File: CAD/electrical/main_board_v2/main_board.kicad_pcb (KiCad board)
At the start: 2 copper layers, 125.2 x 61.2 mm, 70 parts, among them J1 Battery in, J10 I2C Motor, J13 RS485, J14 RS485, J3 Trigger, J301 USB_B, J302 UART PGM, J4 Side select, J7 I2C Peripheral, J8 I2C Peripheral, J9 I2C Motor, Q301 Q_NPN_BEC, Q302 Q_NPN_BEC, SW3 Input encoder, SW301 BOOT, SW302 RESET, U11 SRV05-4, U201 LM2576S-5, U202 AMS1117-3.3, U3 ESP32-WROOM-32, U301 SRV05-4, U302 CP2102N-Axx-xQFN28, U4 PCA9306DC1, U5 PCA9306DC1, U7 LCD-016N002L, U8 MAX485E, U9 SRV05-4

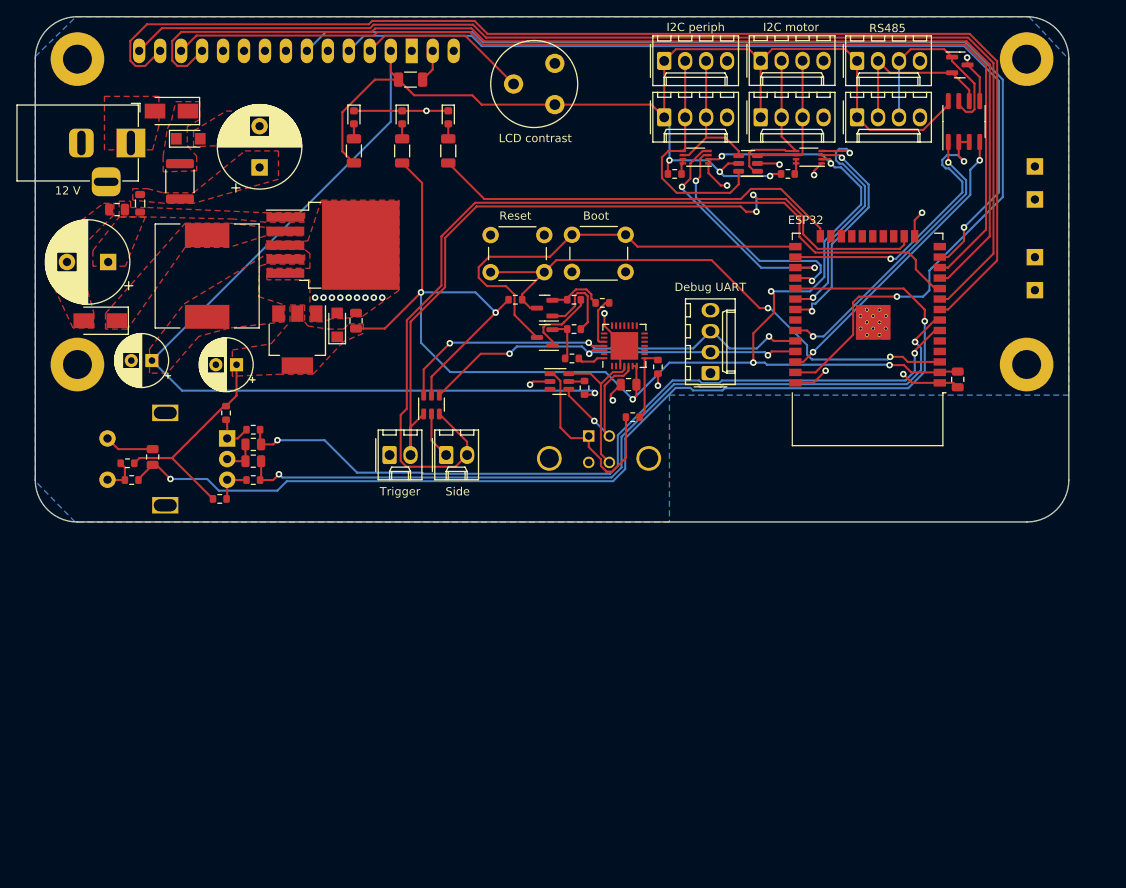
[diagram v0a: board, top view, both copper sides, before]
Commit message: Kicad CAD for mainboard and motorboard (final)
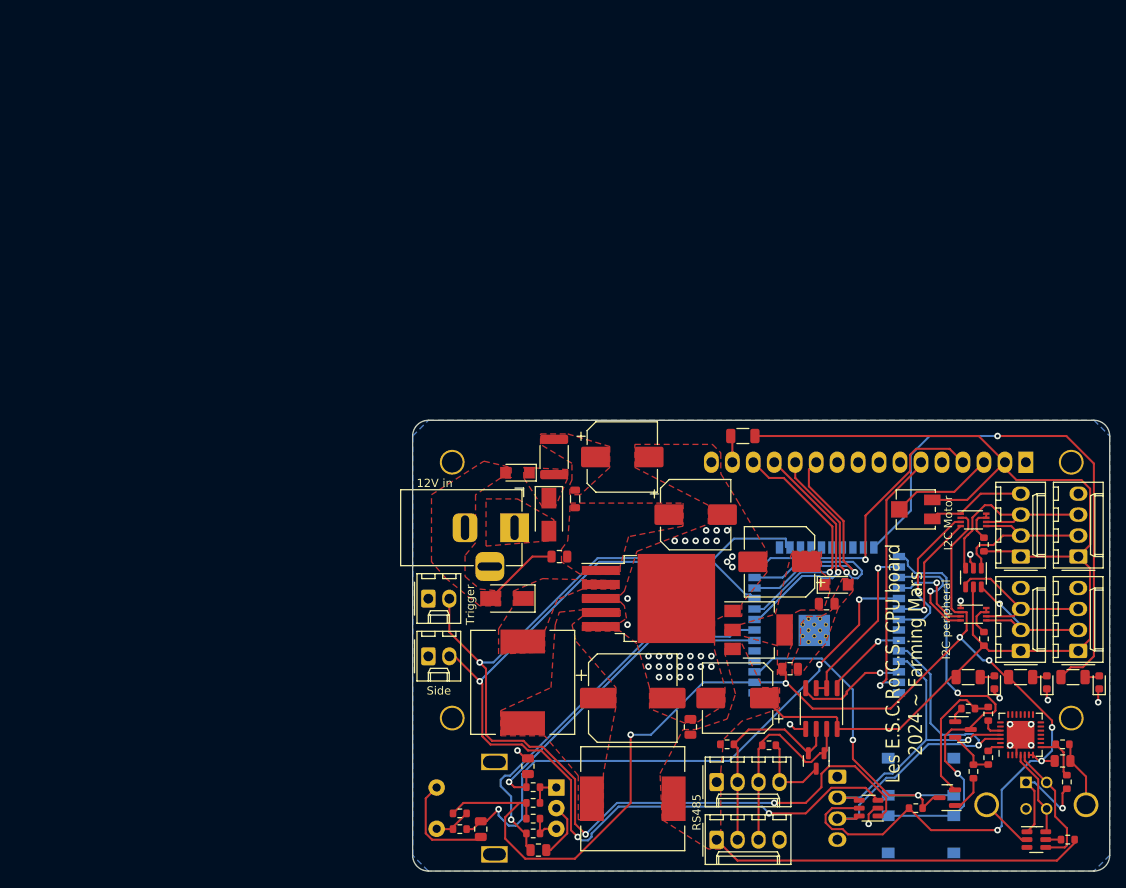
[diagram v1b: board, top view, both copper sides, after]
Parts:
- removed J302: UART PGM, Connector_Molex:Molex_KK-254_AE-6410-04A_1x04_P2.54mm_Vertical
- added C1: 100u, Capacitor_SMD:CP_Elec_8x10, F.Cu at (142.0, 100.1)
- added C2: 100n, Capacitor_SMD:C_0805_2012Metric, F.Cu at (136.3, 103.6)
- added J2: UART PGM, Connector_Molex:Molex_KK-254_AE-6410-04A_1x04_P2.54mm_Vertical, B.Cu at (154.1, 109.6)
- added L1: 10u, Inductor_SMD:L_12x12mm_H6mm, F.Cu at (129.3, 112.3)
- added R2: 1k, Resistor_SMD:R_0603_1608Metric, F.Cu at (140.7, 105.7)
- added R3: 1k, Resistor_SMD:R_0603_1608Metric, F.Cu at (145.8, 105.8)
- C201, C202: footprint Capacitor_THT:CP_Radial_D10.0mm_P5.00mm -> Capacitor_SMD:CP_Elec_8x10
- C204: value 10u -> 2000u; footprint Capacitor_THT:CP_Radial_D6.3mm_P2.50mm -> Capacitor_SMD:CP_Elec_10x10.5
- C205: value 10u -> 100u; footprint Capacitor_THT:CP_Radial_D6.3mm_P2.50mm -> Capacitor_SMD:CP_Elec_8x10
- R1: value 470 -> 300
- R10, R14, R9: value 470 -> 620
- R202, R4: value 100 -> 300
- R301: value 47k -> 82k
- R302: value 24k -> 36k
- R5, R6: value 100k -> 33k
- RV1: footprint Potentiometer_THT:Potentiometer_Piher_PT-10-V05_Vertical -> Potentiometer_SMD:Potentiometer_Bourns_3314J_Vertical
- SW301, SW302: footprint Button_Switch_THT:SW_PUSH_6mm -> Button_Switch_SMD:SW_Push_1P1T_NO_6x6mm_H9.5mm; moved to B.Cu
- U3: footprint RF_Module:ESP32-WROOM-32 -> RF_Module:ESP32-WROOM-32U; moved to B.Cu
- U7: footprint Display:LCD-016N002L -> Display:WC1602A
- moved D4 104.4 mm to (185.8, 98.2), turned to 90 degrees
- moved D205 103.9 mm to (179.5, 98.2), turned to 90 degrees
- moved D204 103.5 mm to (173.1, 98.2), turned to 90 degrees
- moved R4 99.0 mm to (182.6, 97.5), turned to 0 degrees
- moved R202 98.4 mm to (176.3, 97.5), turned to 0 degrees
- moved R201 98.0 mm to (169.9, 97.5), turned to 0 degrees
- moved J13 95.9 mm to (139.4, 117.2)
- moved U7 89.6 mm to (176.9, 71.5)
- moved D8 86.1 mm to (151.5, 107.7), turned to -90 degrees
- moved SW301 84.1 mm to (164.2, 116.6), turned to 180 degrees
- moved SW302 83.8 mm to (164.2, 109.6), turned to 180 degrees
- moved J8 83.5 mm to (176.3, 94.4), turned to 90 degrees
- moved J14 82.3 mm to (139.4, 110.3)
- moved J7 81.8 mm to (183.3, 94.4), turned to 90 degrees
- moved R306 80.1 mm to (182.0, 117.2), turned to 180 degrees
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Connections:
- C204 pad 1: +5V -> Net-(C204-Pad1)
- L201 pad 2: +5V -> Net-(C204-Pad1)
- U201 pad 4: +5V -> Net-(C204-Pad1)
- U3 pad 34: /UART_MOSI -> /UART_RX
- U3 pad 35: /UART_MISO -> /UART_TX
- U302 pad 25: /UART_MOSI -> /UART_TX
- U302 pad 26: /UART_MISO -> /UART_RX
- U9 pad 4: /UART_MISO -> /UART_TX
- U9 pad 6: /UART_MOSI -> /UART_RX
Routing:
- net /LCD_DB6: track 148.6 -> 29.3 mm, vias 0 -> 1
- net /LCD_DB7: track 138.6 -> 29.4 mm, vias 0 -> 1
- net /LCD_E: track 139.5 -> 31.5 mm
- net /LCD_DB4: track 137.5 -> 29.6 mm, vias 0 -> 1
- net /LCD_DB5: track 127.5 -> 32.9 mm, vias 0 -> 1
- net /LCD_RS: track 106.7 -> 36.3 mm
- net /INPUT_SW: track 129.5 -> 71.5 mm, vias 2 -> 3
- net +5V: track 241.9 -> 186.0 mm, vias 4 -> 0
- net /INPUT_A: track 96.3 -> 40.9 mm, vias 2 -> 1
- net /UART_MOSI: track 54.1 -> 0.00 mm, vias 3 -> 0
- net /INPUT_B: track 97.9 -> 48.4 mm, vias 2 -> 1
- net /UART_MISO: track 48.4 -> 0.00 mm, vias 3 -> 0
- net /UART_RX: track 0.00 -> 45.8 mm, vias 0 -> 1
- net /UART_TX: track 0.00 -> 37.2 mm, vias 0 -> 1
- net +3V3: track 210.7 -> 176.8 mm, vias 8 -> 7
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- added copper zone on F.Cu, net Net-(C204-Pad1)
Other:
- board size 125.2 x 61.2 mm -> 84.5 x 54.6 mm
- board text added: "12V in"
- board text added: "BOOT"
- board text added: "I2C Motor"
- board text added: "I2C peripheral"
- board text added: "Les E.S.C.Ro.C.S. CPU board 2024 ~ Farming Mars"
- board text added: "RESET"
- board text added: "UART flash"
- board text removed: "12 V"
- board text removed: "Boot"
- board text removed: "Debug UART"
- board text removed: "ESP32"
- board text removed: "I2C motor"
- board text removed: "I2C periph"
- board text removed: "LCD contrast"
- board text removed: "Reset"
- board text removed: "Rotary encoder"
